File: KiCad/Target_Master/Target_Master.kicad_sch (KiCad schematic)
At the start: 9 parts, among them J1 RJ11 Header, U2 PIC16F1788-IP

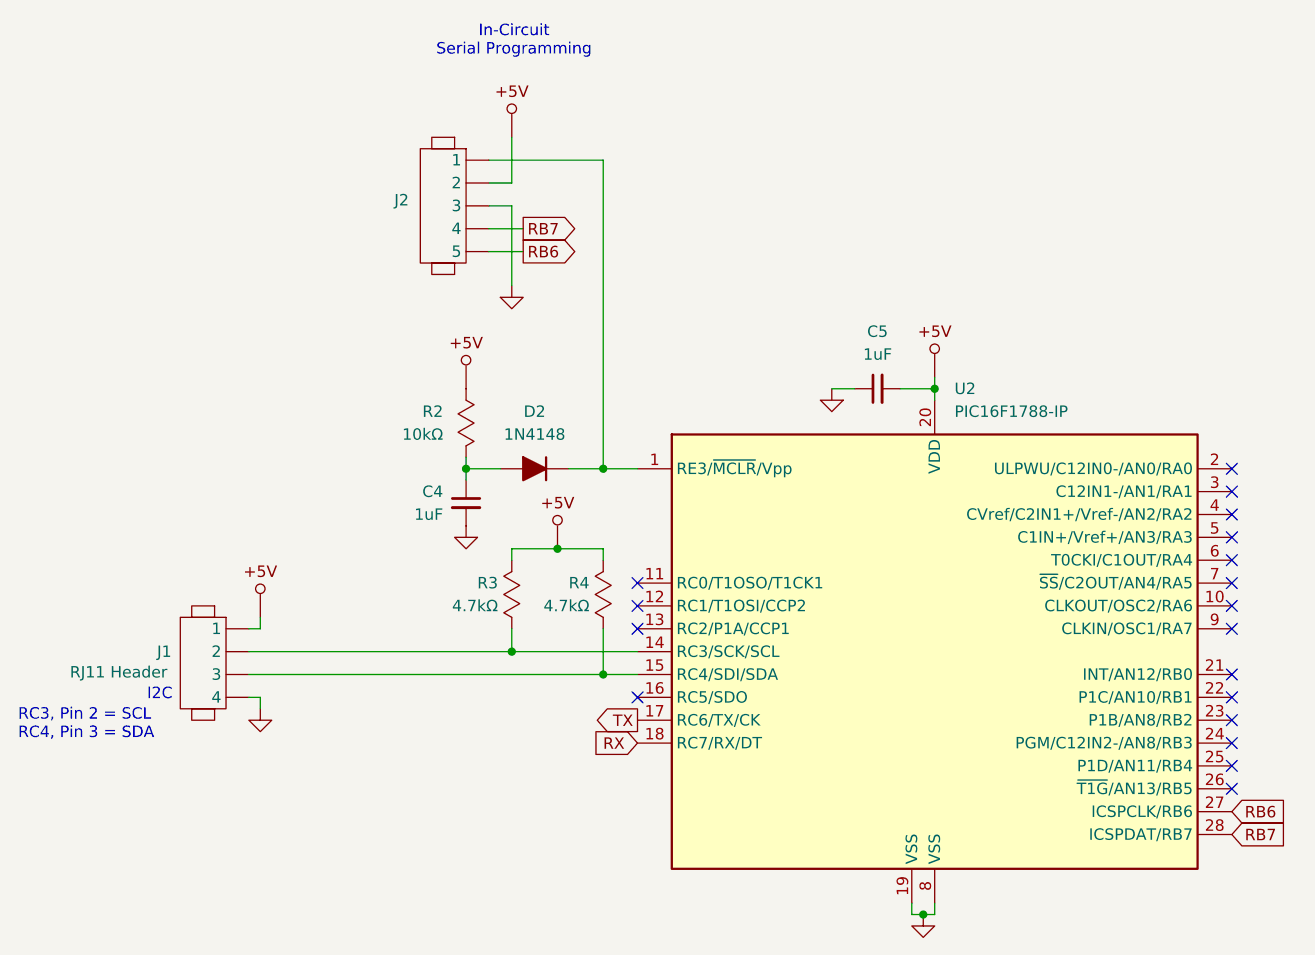
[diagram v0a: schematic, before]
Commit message: Finalized schematics
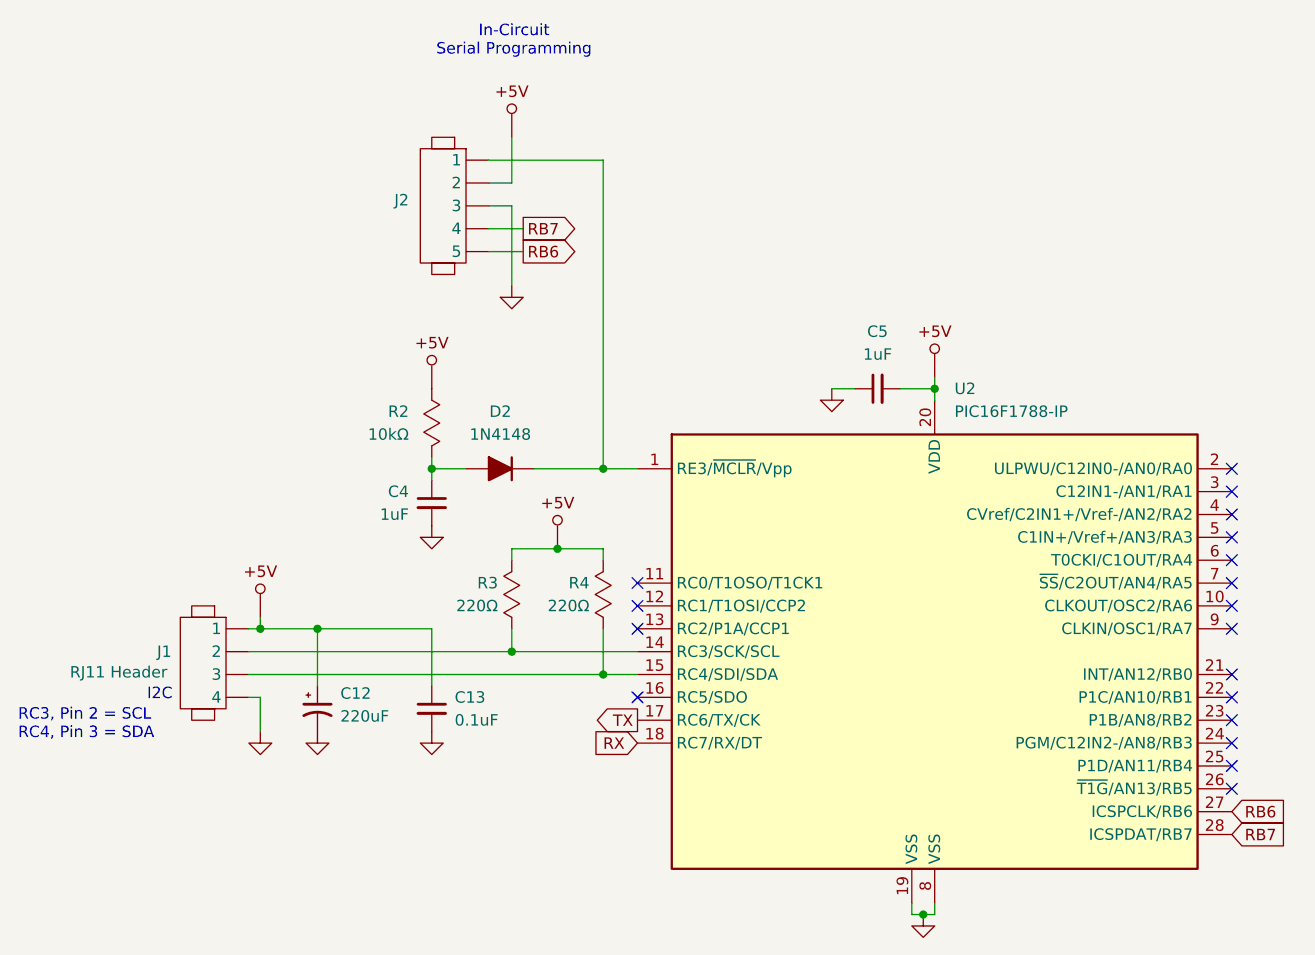
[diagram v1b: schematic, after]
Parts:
- added C12: 220uF, symbol Device:C_Polarized_Small_US
- added C13: 0.1uF, symbol Device:C_Small
- R3, R4: value 4.7kΩ -> 220Ω
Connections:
- net +5V: now also C12.1, C13.1
- net GND: now also C12.2, C13.2
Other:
- moved on the sheet: C4, D2, R2
